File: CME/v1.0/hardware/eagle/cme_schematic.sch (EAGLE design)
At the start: 15 parts, among them T1 BC547, T2 BC547

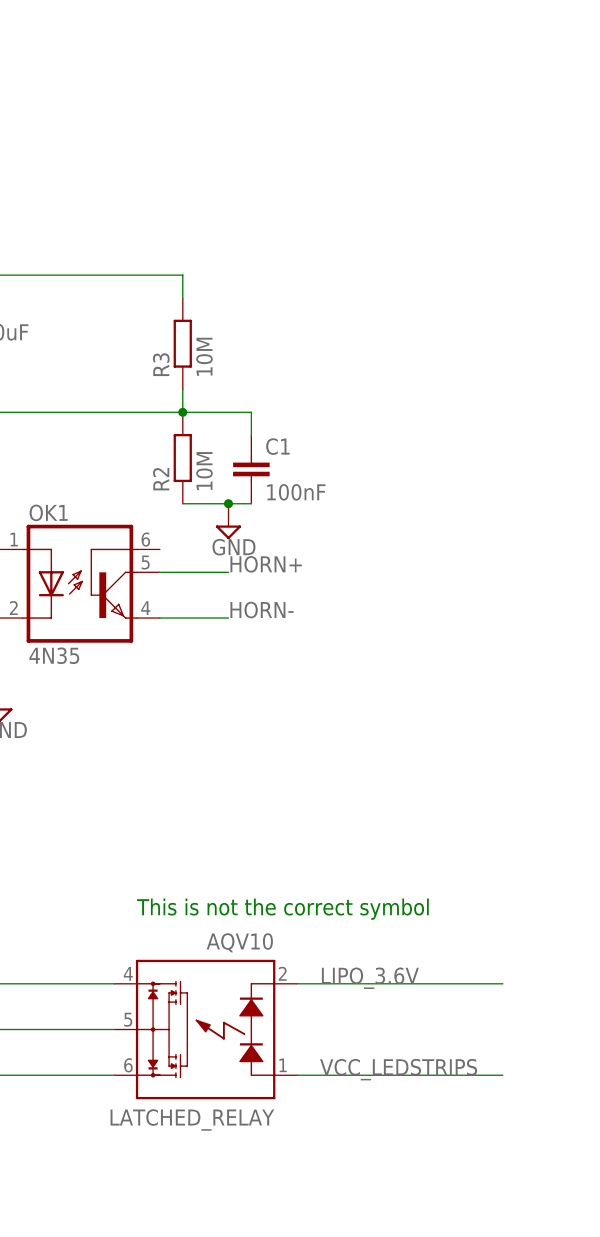
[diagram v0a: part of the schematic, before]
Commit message: updated schematic
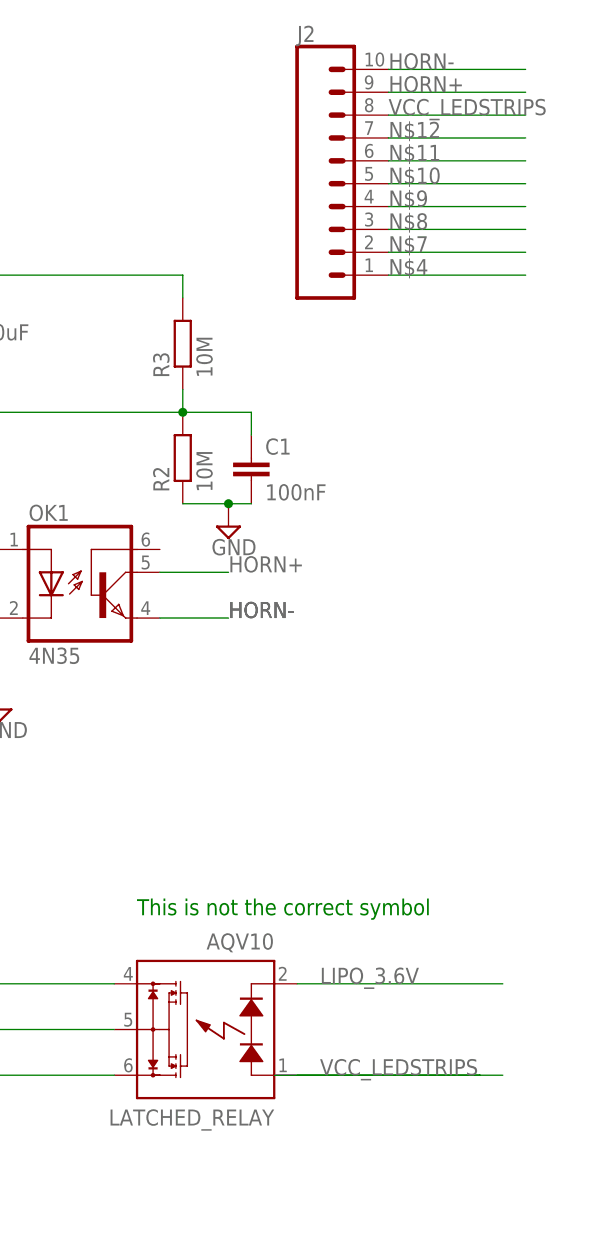
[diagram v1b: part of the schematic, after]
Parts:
- added J2: (no value), SparkFun-Connectors:CONN_10"
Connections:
- new net N$10: J2.5
- new net N$11: J2.6
- new net N$12: J2.7
- new net N$14: J2.9
- new net N$15: J2.10
- new net N$4: J2.1
- new net N$7: J2.2
- new net N$8: J2.3
- new net N$9: J2.4
- net VCC_LEDSTRIPS: now also J2.8
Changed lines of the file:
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@@
 <part name="D1" library="diode" library_urn="urn:adsk.eagle:library:210" deviceset="1N4004" device="" package3d_urn="urn:adsk.eagle:package:43336/1"/>
 <part name="D2" library="diode" library_urn="urn:adsk.eagle:library:210" deviceset="1N4004" device="" package3d_urn="urn:adsk.eagle:package:43336/1"/>
+<part name="J2" library="SparkFun-Connectors" library_urn="urn:adsk.eagle:library:513" deviceset="CONN_10" device="&quot;" package3d_urn="urn:adsk.eagle:package:38157/1"/>
 </parts>
 <sheets>
@@
 <attribute name="NAME" x="60.4774" y="-7.62" size="1.778" layer="95" rot="R90"/>
 <attribute name="VALUE" x="63.2714" y="-7.62" size="1.778" layer="96" rot="R90"/>
+</instance>
+<instance part="J2" gate="G$1" x="121.92" y="81.28" smashed="yes">
+<attribute name="VALUE" x="121.92" y="58.674" size="1.778" layer="96" font="vector"/>
+<attribute name="NAME" x="121.92" y="89.408" size="1.778" layer="95" font="vector"/>
 </instance>
 </instances>
@@
 <wire x1="106.68" y1="30.48" x2="114.3" y2="30.48" width="0.1524" layer="91"/>
 <label x="114.3" y="30.48" size="1.778" layer="95"/>
+<label x="132.08" y="83.82" size="1.778" layer="95"/>
 </segment>
 </net>
@@
 <wire x1="106.68" y1="25.4" x2="114.3" y2="25.4" width="0.1524" layer="91"/>
 <label x="114.3" y="25.4" size="1.778" layer="95"/>
+<label x="114.3" y="25.4" size="1.778" layer="95"/>
+<label x="132.08" y="86.36" size="1.778" layer="95"/>
 </segment>
 </net>
@@
 <segment>
 <pinref part="LATCHED_RELAY" gate="G$1" pin="A"/>
-<wire x1="121.92" y1="-25.4" x2="144.78" y2="-25.4" width="0.1524" layer="91"/>
+<wire x1="121.92" y1="-25.4" x2="142.24" y2="-25.4" width="0.1524" layer="91"/>
 <label x="124.46" y="-25.4" size="1.778" layer="95"/>
+<wire x1="142.24" y1="-25.4" x2="144.78" y2="-25.4" width="0.1524" layer="91"/>
+<wire x1="119.38" y1="-25.4" x2="142.24" y2="-25.4" width="0.1524" layer="91"/>
+</segment>
+<segment>
+<pinref part="J2" gate="G$1" pin="8"/>
+<wire x1="132.08" y1="81.28" x2="147.32" y2="81.28" width="0.1524" layer="91"/>
+<label x="132.08" y="81.28" size="1.778" layer="95"/>
 </segment>
 </net>
@@
 </segment>
 </net>
+<net name="N$4" class="0">
+<segment>
+<pinref part="J2" gate="G$1" pin="1"/>
+<wire x1="132.08" y1="63.5" x2="147.32" y2="63.5" width="0.1524" layer="91"/>
+<label x="132.08" y="63.5" size="1.778" layer="95"/>
+</segment>
+</net>
+<net name="N$7" class="0">
+<segment>
+<pinref part="J2" gate="G$1" pin="2"/>
+<wire x1="132.08" y1="66.04" x2="147.32" y2="66.04" width="0.1524" layer="91"/>
+<label x="132.08" y="66.04" size="1.778" layer="95"/>
+</segment>
+</net>
+<net name="N$8" class="0">
+<segment>
+<pinref part="J2" gate="G$1" pin="3"/>
+<wire x1="132.08" y1="68.58" x2="147.32" y2="68.58" width="0.1524" layer="91"/>
+<label x="132.08" y="68.58" size="1.778" layer="95"/>
+</segment>
+</net>
+<net name="N$9" class="0">
+<segment>
+<pinref part="J2" gate="G$1" pin="4"/>
+<wire x1="132.08" y1="71.12" x2="147.32" y2="71.12" width="0.1524" layer="91"/>
+<label x="132.08" y="71.12" size="1.778" layer="95"/>
+</segment>
+</net>
+<net name="N$10" class="0">
+<segment>
+<pinref part="J2" gate="G$1" pin="5"/>
+<wire x1="132.08" y1="73.66" x2="147.32" y2="73.66" width="0.1524" layer="91"/>
+<label x="132.08" y="73.66" size="1.778" layer="95"/>
+</segment>
+</net>
+<net name="N$11" class="0">
+<segment>
+<pinref part="J2" gate="G$1" pin="6"/>
+<wire x1="132.08" y1="76.2" x2="147.32" y2="76.2" width="0.1524" layer="91"/>
+<label x="132.08" y="76.2" size="1.778" layer="95"/>
+</segment>
+</net>
+<net name="N$12" class="0">
+<segment>
+<pinref part="J2" gate="G$1" pin="7"/>
+<wire x1="132.08" y1="78.74" x2="147.32" y2="78.74" width="0.1524" layer="91"/>
+<label x="132.08" y="78.74" size="1.778" layer="95"/>
+</segment>
+</net>
+<net name="N$14" class="0">
+<segment>
+<pinref part="J2" gate="G$1" pin="9"/>
+<wire x1="132.08" y1="83.82" x2="147.32" y2="83.82" width="0.1524" layer="91"/>
+</segment>
+</net>
+<net name="N$15" class="0">
+<segment>
+<pinref part="J2" gate="G$1" pin="10"/>
+<wire x1="132.08" y1="86.36" x2="147.32" y2="86.36" width="0.1524" layer="91"/>
+</segment>
+</net>
